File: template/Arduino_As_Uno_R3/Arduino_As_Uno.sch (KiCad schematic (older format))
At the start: 4 parts, among them P1 Power, P2 Analog, P3 Digital, P4 Digital

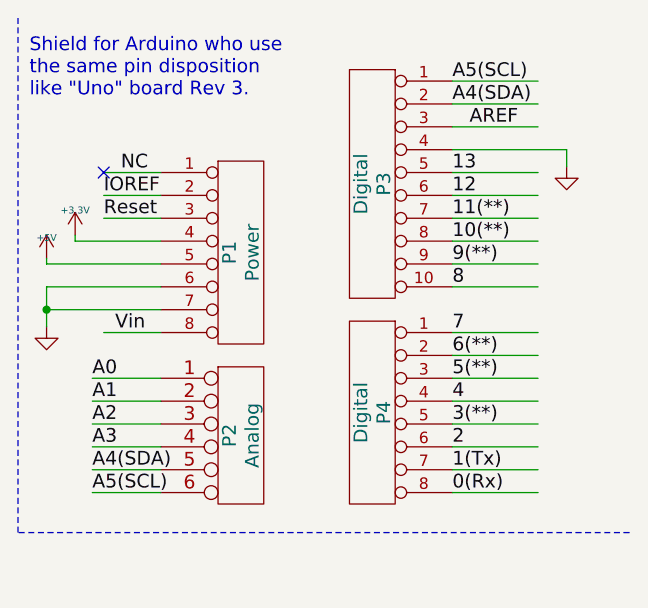
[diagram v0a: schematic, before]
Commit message: correction holes
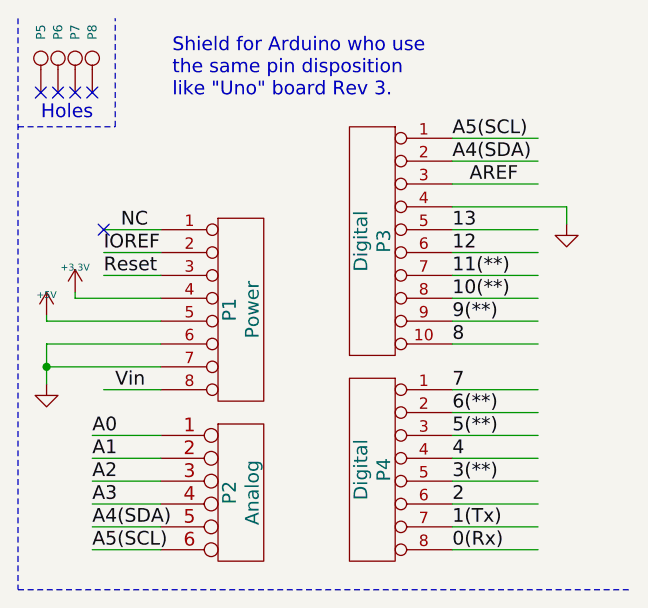
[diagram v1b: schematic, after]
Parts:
- added P5, P6, P7, P8: CONN_1, Connect:1pin, symbol CONN_1
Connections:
- no-connect marks 1 -> 5
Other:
- note added: "Holes"
- moved on the sheet: P1, P2, P3, P4
